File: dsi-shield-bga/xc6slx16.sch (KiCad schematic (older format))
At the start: 15 parts, among them IC2 M25P80-VMN6P, IC3 25MHz, U1 XC6SLX16-FTG256

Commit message: 20200808
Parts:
- added R36: 1k, Resistor_SMD:R_0402_1005Metric, symbol dsi_shield:Res1
- added R40: 100, Resistor_SMD:R_0402_1005Metric, symbol dsi_shield:Res1
- IC2: footprint Package_SO:SOIC-8_7.5x5.85mm_P1.27mm -> Package_DFN_QFN:DFN-8-1EP_6x5mm_P1.27mm_EP4x4mm
- IC3: footprint Oscillator:Oscillator_SMD_EuroQuartz_XO53-4Pin_5.0x3.2mm -> Oscillator:Oscillator_SMD_Abracon_ASE-4Pin_3.2x2.5mm_HandSoldering
- R31: value 0 -> 1k
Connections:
- net labels added: +3.3V, DDR_VREF, FPGA_M0, FPGA_TCK, FPGA_TDI, FPGA_TDO, FPGA_TMS, HPD_NOTIFY, QSPI_CLK, QSPI_CS0, QSPI_DQ0, QSPI_DQ1, QSPI_DQ2, QSPI_DQ3, SCL, SDA, SDRAM_A[0..14], SDRAM_BA0, SDRAM_BA1, SDRAM_BA[0..1], SDRAM_CLK_N, SDRAM_CLK_P, SDRAM_CS_N, SDRAM_DQS0, SDRAM_DQS1, SDRAM_DQS[0..1], V_DDR
- net labels removed: +2V5, CFG_CLK, CFG_CS0, CFG_M0, CFG_MISO, CFG_MOSI, DSI_HS_N0, DSI_HS_N1, DSI_HS_N2, DSI_HS_N3, DSI_HS_P0, DSI_HS_P1, DSI_HS_P2, DSI_HS_P3, DSI_LP_N0, DSI_LP_N1, DSI_LP_N2, DSI_LP_N3, DSI_LP_P0, DSI_LP_P1, DSI_LP_P2, DSI_LP_P3, FGPA_SCL, FPGA_SDA, HPD_NOTIF, SDRAM_A[0..12], TCK, TDI, TDO, TMS
- wire segments 275 -> 367
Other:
- moved on the sheet: C18, C19, D5, IC2, IC3, R26, R27, R28, R29, R30, R31, R32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

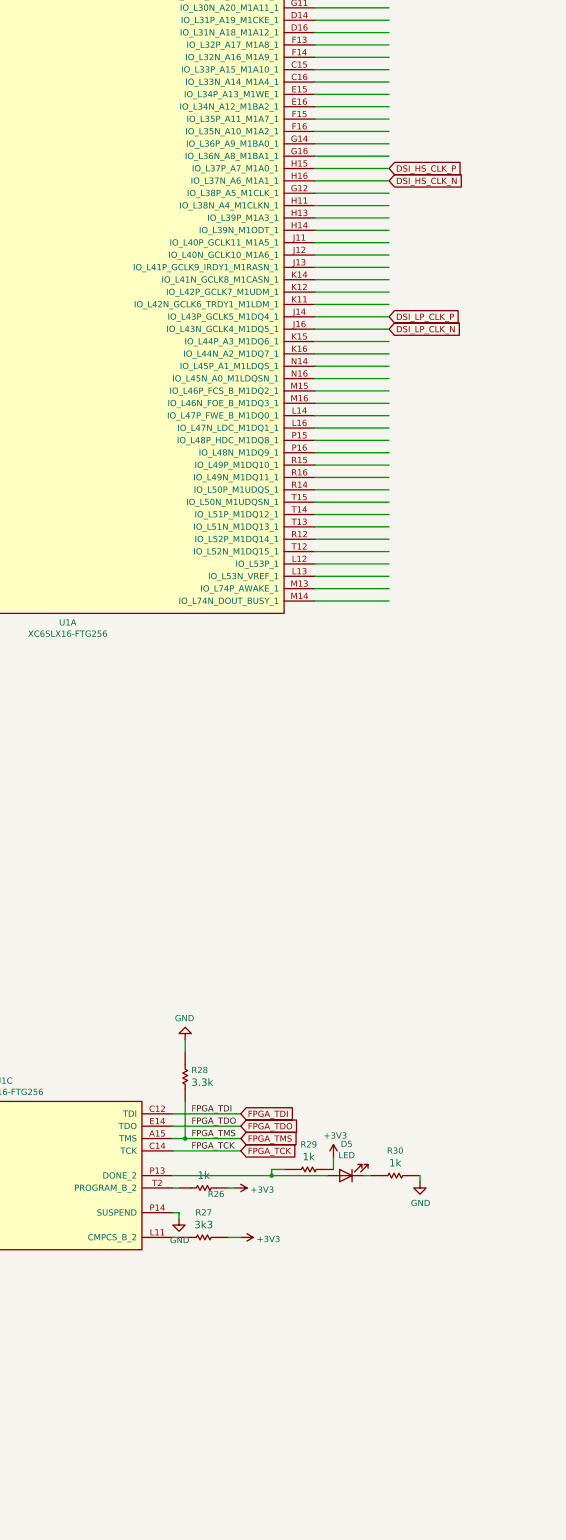
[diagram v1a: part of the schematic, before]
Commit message: pin head
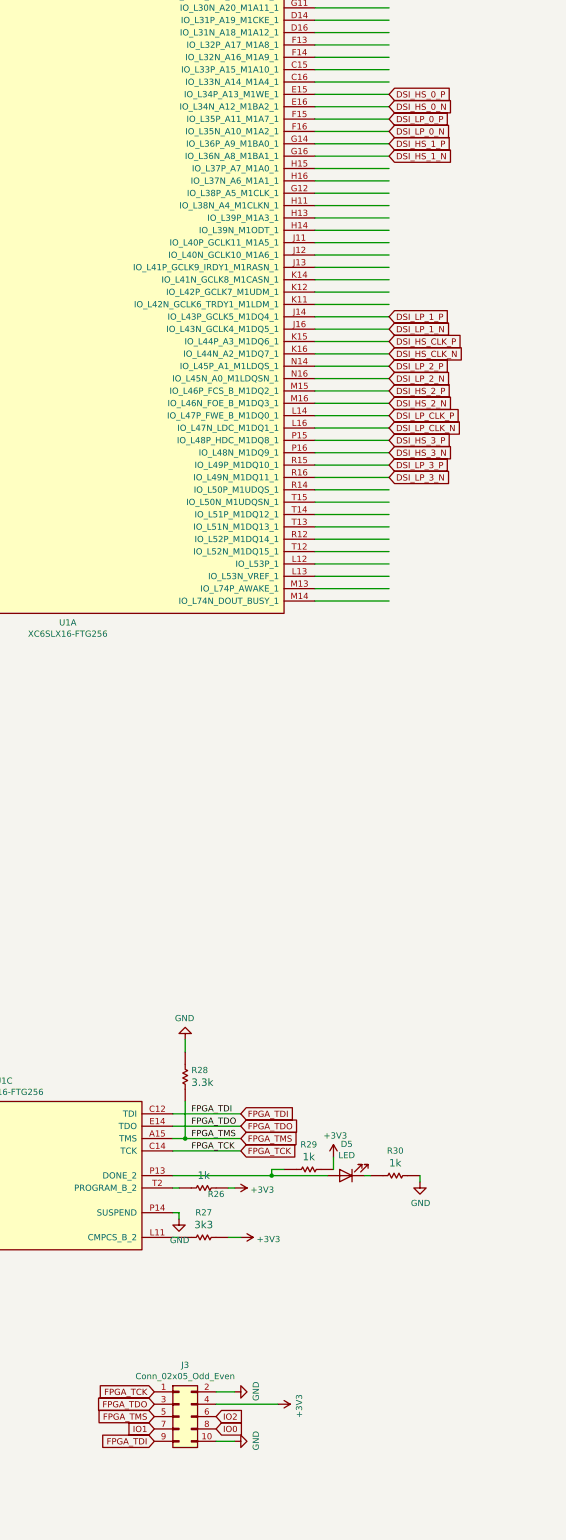
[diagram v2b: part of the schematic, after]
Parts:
- added J3: Conn_02x05_Odd_Even, mybays_connector:debugger_2x05_P1.27mm_Vertical, symbol Connector_Generic:Conn_02x05_Odd_Even
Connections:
- net labels added: DSI_HS_0_N, DSI_HS_0_P, DSI_HS_1_N, DSI_HS_1_P, DSI_HS_2_N, DSI_HS_2_P, DSI_HS_3_N, DSI_HS_3_P, DSI_LP_0_N, DSI_LP_0_P, DSI_LP_1_N, DSI_LP_1_P, DSI_LP_2_N, DSI_LP_2_P, DSI_LP_3_N, DSI_LP_3_P, IO0, IO1, IO2
- wire segments 367 -> 370
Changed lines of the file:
@@
 Text HLabel 1050 3450 0    50   Input ~ 0
 DBG_RX
-Text GLabel 6150 3750 2    50   Input ~ 0
+Text GLabel 6150 5150 2    50   Input ~ 0
 DSI_HS_CLK_P
-Text GLabel 6150 3850 2    50   Input ~ 0
+Text GLabel 6150 5250 2    50   Input ~ 0
 DSI_HS_CLK_N
 $Comp
@@
 	1    0    0    -1
 $EndComp
+Text GLabel 6150 5850 2    50   Input ~ 0
+DSI_LP_CLK_N
+Text GLabel 6150 5750 2    50   Input ~ 0
+DSI_LP_CLK_P
+$Comp
+L Connector_Generic:Conn_02x05_Odd_Even J3
+U 1 1 5F33AAA6
+P 4450 13850
+F 0 "J3" H 4500 14267 50  0000 C CNN
+F 1 "Conn_02x05_Odd_Even" H 4500 14176 50  0000 C CNN
+F 2 "mybays_connector:debugger_2x05_P1.27mm_Vertical" H 4450 13850 50  0001 C CNN
+F 3 "~" H 4450 13850 50  0001 C CNN
+	1    4450 13850
+	1    0    0    -1
+$EndComp
+Text GLabel 4250 13650 0    50   Input ~ 0
+FPGA_TCK
+Text GLabel 4250 13750 0    50   Input ~ 0
+FPGA_TDO
+Text GLabel 4250 13850 0    50   Input ~ 0
+FPGA_TMS
+Text GLabel 4250 14050 0    50   Input ~ 0
+FPGA_TDI
+$Comp
+L power:GND #PWR0194
+U 1 1 5F3413B0
+P 4900 13650
+F 0 "#PWR0194" H 4900 13400 50  0001 C CNN
+F 1 "GND" H 4905 13477 50  0000 C CNN
+F 2 "" H 4900 13650 50  0001 C CNN
+F 3 "" H 4900 13650 50  0001 C CNN
+	1    4900 13650
+	0    -1   -1   0
+$EndComp
+$Comp
+L power:GND #PWR0195
+U 1 1 5F341C21
+P 4900 14050
+F 0 "#PWR0195" H 4900 13800 50  0001 C CNN
+F 1 "GND" H 4905 13877 50  0000 C CNN
+F 2 "" H 4900 14050 50  0001 C CNN
+F 3 "" H 4900 14050 50  0001 C CNN
+	1    4900 14050
+	0    -1   -1   0
+$EndComp
+$Comp
+L power:+3V3 #PWR0196
+U 1 1 5F3449ED
+P 5250 13750
+F 0 "#PWR0196" H 5250 13600 50  0001 C CNN
+F 1 "+3V3" H 5265 13923 50  0000 C CNN
+F 2 "" H 5250 13750 50  0001 C CNN
+F 3 "" H 5250 13750 50  0001 C CNN
+	1    5250 13750
+	0    1    1    0
+$EndComp
+Wire Wire Line
+	4750 13650 4900 13650
+Wire Wire Line
+	4750 13750 5250 13750
+Wire Wire Line
+	4750 14050 4900 14050
+Text GLabel 4250 13950 0    50   Input ~ 0
+IO1
+Text GLabel 4750 13950 2    50   Input ~ 0
+IO0
+Text GLabel 4750 13850 2    50   Input ~ 0
+IO2
+Text GLabel 6150 6250 2    50   Input ~ 0
+DSI_LP_3_N
+Text GLabel 6150 6150 2    50   Input ~ 0
+DSI_LP_3_P
+Text GLabel 6150 6050 2    50   Input ~ 0
+DSI_HS_3_N
+Text GLabel 6150 5950 2    50   Input ~ 0
+DSI_HS_3_P
+Text GLabel 6150 5450 2    50   Input ~ 0
+DSI_LP_2_N
+Text GLabel 6150 5350 2    50   Input ~ 0
+DSI_LP_2_P
+Text GLabel 6150 5650 2    50   Input ~ 0
+DSI_HS_2_N
+Text GLabel 6150 5550 2    50   Input ~ 0
+DSI_HS_2_P
 Text GLabel 6150 5050 2    50   Input ~ 0
-DSI_LP_CLK_N
+DSI_LP_1_N
 Text GLabel 6150 4950 2    50   Input ~ 0
-DSI_LP_CLK_P
+DSI_LP_1_P
+Text GLabel 6150 3650 2    50   Input ~ 0
+DSI_HS_1_N
+Text GLabel 6150 3550 2    50   Input ~ 0
+DSI_HS_1_P
+Text GLabel 6150 3450 2    50   Input ~ 0
+DSI_LP_0_N
+Text GLabel 6150 3350 2    50   Input ~ 0
+DSI_LP_0_P
+Text GLabel 6150 3250 2    50   Input ~ 0
+DSI_HS_0_N
+Text GLabel 6150 3150 2    50   Input ~ 0
+DSI_HS_0_P
 Wire Bus Line
 	19700 4450 19700 4600
